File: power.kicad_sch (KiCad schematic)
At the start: 16 parts, among them IC1 TPS63070RNMR

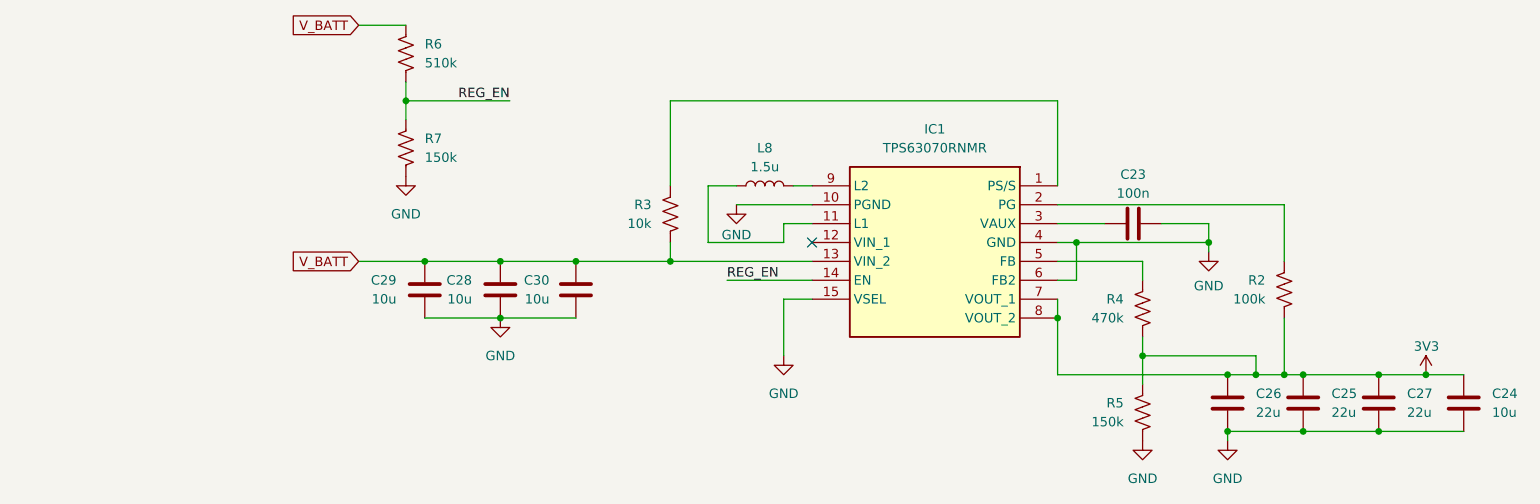
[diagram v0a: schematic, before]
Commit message: proper formating
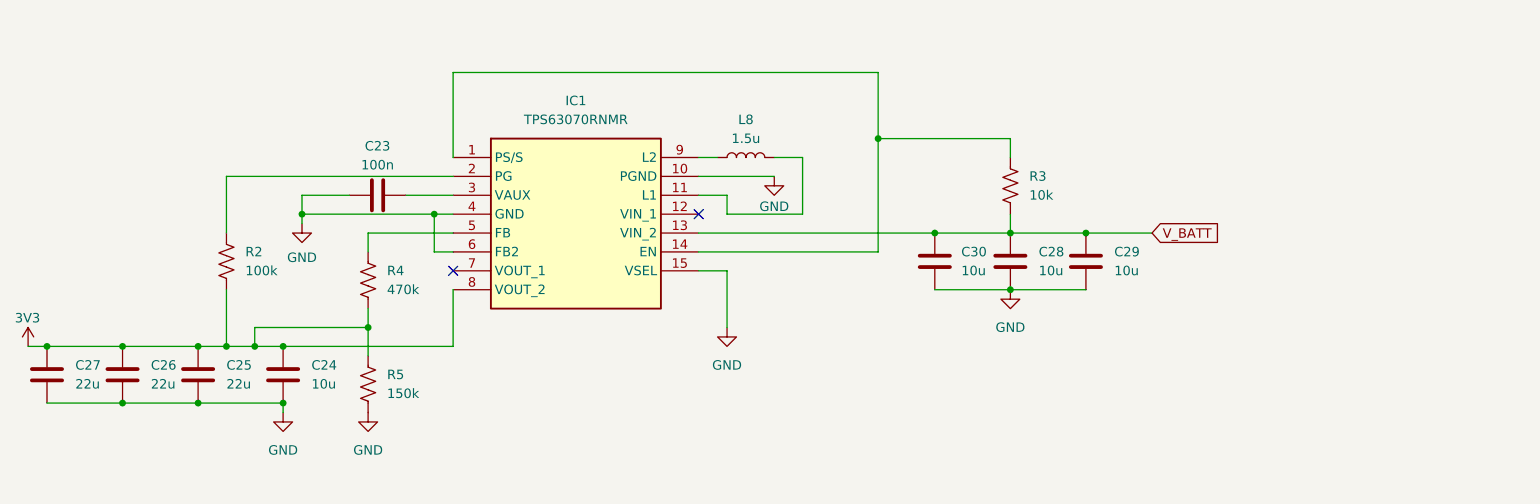
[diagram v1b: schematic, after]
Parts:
- removed R6: 510k, symbol Device:R_US
- removed R7: 150k, symbol Device:R_US
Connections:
- net REG_EN is gone; now on an unnamed net: IC1.14 (EN)
- net 3V3: no longer IC1.7 (VOUT_1)
- no-connect marks 1 -> 2
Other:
- moved on the sheet: C23, C24, C25, C26, C28, C29, C30, IC1, L8, R2, R3, R4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
